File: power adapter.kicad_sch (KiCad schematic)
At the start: 8 parts

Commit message: added mfp#for header
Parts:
- U1: manFp# (none) -> CONN HEADER VERT 10POS 2.54MM
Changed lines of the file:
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@@
+			)
+		)
+		(property "manFp#" "CONN HEADER VERT 10POS 2.54MM"
+			(at 21.59 41.91 0)
+			(effects
+				(font
+					(size 1.27 1.27)
+				)
+				(hide yes)
 			)
 		)

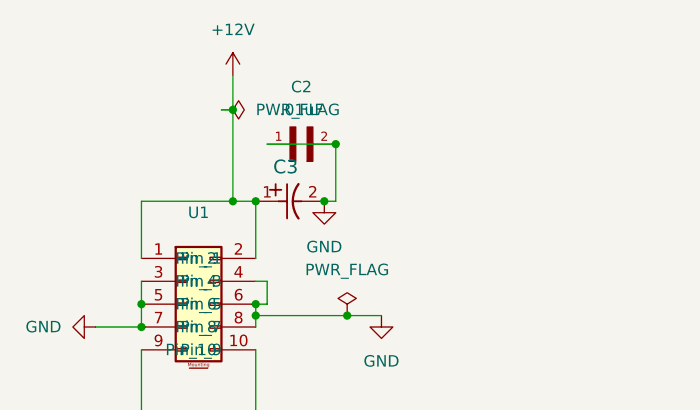
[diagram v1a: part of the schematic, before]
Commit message: fixedc2
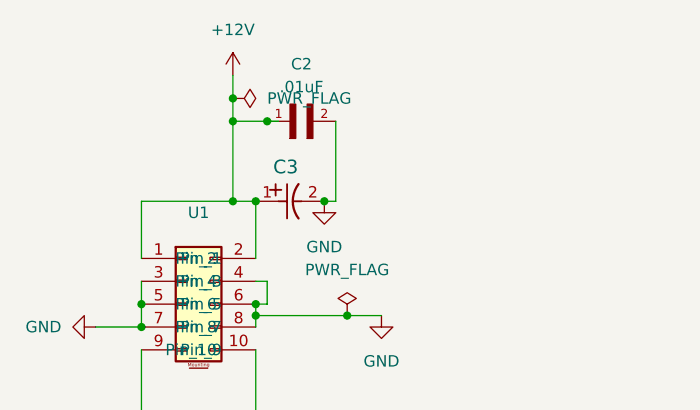
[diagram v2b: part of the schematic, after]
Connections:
- net +12V: now also C2.1
- net GND: no longer C2.1
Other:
- moved on the sheet: C2
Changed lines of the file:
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@@
 	(paper "A4")
-	(junction
-		(at 31.75 26.67)
-		(diameter 0)
-		(color 0 0 0 0)
-	)
 	(junction
 		(at 44.45 49.53)
@@
 	)
 	(junction
-		(at 43.18 30.48)
+		(at 34.29 68.58)
 		(diameter 0)
 		(color 0 0 0 0)
 	)
 	(junction
-		(at 34.29 68.58)
+		(at 31.75 27.94)
 		(diameter 0)
 		(color 0 0 0 0)
@@
 	)
 	(junction
+		(at 31.75 25.4)
+		(diameter 0)
+		(color 0 0 0 0)
+	)
+	(junction
 		(at 41.91 36.83)
 		(diameter 0)
@@
 	)
 	(junction
+		(at 35.56 27.94)
+		(diameter 0)
+		(color 0 0 0 0)
+	)
+	(junction
 		(at 34.29 62.23)
 		(diameter 0)
@@
 	(wire
 		(pts
-			(xy 31.75 22.86) (xy 31.75 26.67)
+			(xy 35.56 27.94) (xy 31.75 27.94)
 		)
 		(stroke
@@
 	(wire
 		(pts
-			(xy 43.18 30.48) (xy 43.18 36.83)
-		)
-		(stroke
-			(width 0)
-			(type default)
-		)
-	)
-	(wire
-		(pts
 			(xy 35.56 45.72) (xy 35.56 48.26)
 		)
@@
 	(wire
 		(pts
-			(xy 31.75 26.67) (xy 31.75 36.83)
+			(xy 31.75 22.86) (xy 31.75 25.4)
 		)
 		(stroke
@@
 	(wire
 		(pts
+			(xy 31.75 25.4) (xy 31.75 27.94)
+		)
+		(stroke
+			(width 0)
+			(type default)
+		)
+	)
+	(wire
+		(pts
 			(xy 34.29 63.5) (xy 34.29 68.58)
 		)
@@
 	(wire
 		(pts
+			(xy 31.75 27.94) (xy 31.75 36.83)
+		)
+		(stroke
+			(width 0)
+			(type default)
+		)
+	)
+	(wire
+		(pts
 			(xy 34.29 36.83) (xy 34.29 43.18)
 		)
@@
 	(wire
 		(pts
+			(xy 35.56 27.94) (xy 36.83 27.94)
+		)
+		(stroke
+			(width 0)
+			(type default)
+		)
+	)
+	(wire
+		(pts
+			(xy 43.18 27.94) (xy 43.18 36.83)
+		)
+		(stroke
+			(width 0)
+			(type default)
+		)
+	)
+	(wire
+		(pts
 			(xy 34.29 77.47) (xy 44.45 77.47)
 		)
@@
 	(wire
 		(pts
-			(xy 35.56 30.48) (xy 43.18 30.48)
-		)
-		(stroke
-			(width 0)
-			(type default)
-		)
-	)
-	(wire
-		(pts
 			(xy 21.59 63.5) (xy 31.75 63.5)
 		)
@@
 		(pts
 			(xy 21.59 48.26) (xy 21.59 50.8)
-		)
-		(stroke
-			(width 0)
-			(type default)
-		)
-	)
-	(wire
-		(pts
-			(xy 31.75 26.67) (xy 30.48 26.67)
 		)
 		(stroke
@@
 	(symbol
 		(lib_id "power:PWR_FLAG")
-		(at 30.48 26.67 270)
+		(at 31.75 25.4 270)
 		(unit 1)
 		(exclude_from_sim no)
@@
 		(fields_autoplaced yes)
 		(property "Reference" "#FLG2"
-			(at 32.385 26.67 0)
+			(at 33.655 25.4 0)
 			(effects
 				(font
@@
 		)
 		(property "Value" "PWR_FLAG"
-			(at 34.29 26.6699 90)
+			(at 35.56 25.3999 90)
 			(effects
 				(font
@@
 		)
 		(property "Footprint" ""
-			(at 30.48 26.67 0)
+			(at 31.75 25.4 0)
 			(effects
 				(font
@@
 		)
 		(property "Datasheet" "~"
-			(at 30.48 26.67 0)
+			(at 31.75 25.4 0)
 			(effects
 				(font
@@
 		)
 		(property "Description" "Special symbol for telling ERC where power comes from"
-			(at 30.48 26.67 0)
+			(at 31.75 25.4 0)
 			(effects
 				(font
@@
 	(symbol
 		(lib_id "adapterlib:ceramiccap")
-		(at 38.1 30.48 0)
+		(at 38.1 27.94 0)
 		(unit 1)
 		(exclude_from_sim no)
@@
 		(fields_autoplaced yes)
 		(property "Reference" "C2"
+			(at 39.37 21.59 0)
+			(effects
+				(font
+					(size 1.27 1.27)
+				)
+			)
+		)
+		(property "Value" ".01uF"
 			(at 39.37 24.13 0)
 			(effects
@@
 			)
 		)
-		(property "Value" ".01uF"
-			(at 39.37 26.67 0)
-			(effects
-				(font
-					(size 1.27 1.27)
-				)
-			)
-		)
 		(property "Footprint" "adpterpcblib:CAPC1608X90N"
-			(at 38.1 30.48 0)
+			(at 38.1 27.94 0)
 			(effects
 				(font
@@
 		)
 		(property "Datasheet" ""
-			(at 38.1 30.48 0)
+			(at 38.1 27.94 0)
 			(effects
 				(font
@@
 		)
 		(property "Description" ""
-			(at 38.1 30.48 0)
+			(at 38.1 27.94 0)
 			(effects
 				(font
@@
 		)
 		(property "E_max" "0.9"
-			(at 38.1 30.48 0)
+			(at 38.1 27.94 0)
 			(effects
 				(font
@@
 		)
 		(property "L_max" "0.5"
-			(at 38.1 30.48 0)
+			(at 38.1 27.94 0)
 			(effects
 				(font
@@
 		)
 		(property "A_max" "0.9"
-			(at 38.1 30.48 0)
+			(at 38.1 27.94 0)
 			(effects
 				(font
@@
 		)
 		(property "L1_nom" "0.3"
-			(at 38.1 30.48 0)
+			(at 38.1 27.94 0)
 			(effects
 				(font
@@
 		)
 		(property "D_max" "1.7"
-			(at 38.1 30.48 0)
+			(at 38.1 27.94 0)
 			(effects
 				(font
@@
 		)
 		(property "A_nom" "0.9"
-			(at 38.1 30.48 0)
+			(at 38.1 27.94 0)
 			(effects
 				(font
@@
 		)
 		(property "L1_max" "0.5"
-			(at 38.1 30.48 0)
+			(at 38.1 27.94 0)
 			(effects
 				(font
@@
 		)
 		(property "L1_min" "0.1"
-			(at 38.1 30.48 0)
+			(at 38.1 27.94 0)
 			(effects
 				(font
@@
 		)
 		(property "A_min" "0.9"
-			(at 38.1 30.48 0)
+			(at 38.1 27.94 0)
 			(effects
 				(font
@@
 		)
 		(property "E_min" "0.7"
-			(at 38.1 30.48 0)
+			(at 38.1 27.94 0)
 			(effects
 				(font
@@
 		)
 		(property "D_min" "1.5"
-			(at 38.1 30.48 0)
+			(at 38.1 27.94 0)
 			(effects
 				(font
@@
 		)
 		(property "D_nom" "1.6"
-			(at 38.1 30.48 0)
+			(at 38.1 27.94 0)
 			(effects
 				(font
@@
 		)
 		(property "E_nom" "0.8"
-			(at 38.1 30.48 0)
+			(at 38.1 27.94 0)
 			(effects
 				(font
@@
 		)
 		(property "STANDARD" "IPC 7351B"
-			(at 38.1 30.48 0)
+			(at 38.1 27.94 0)
 			(effects
 				(font
@@
 		)
 		(property "L_min" "0.1"
-			(at 38.1 30.48 0)
+			(at 38.1 27.94 0)
 			(effects
 				(font
@@
 		)
 		(property "L_nom" "0.3"
-			(at 38.1 30.48 0)
+			(at 38.1 27.94 0)
 			(effects
 				(font
@@
 		)
 		(property "MANUFACTURER" "Samsung Electro-Mechanics"
-			(at 38.1 30.48 0)
-			(effects
-				(font
+			(at 38.1 27.94 0)
+			(effects
+				(font
